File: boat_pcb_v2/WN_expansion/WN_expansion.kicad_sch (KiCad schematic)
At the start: 3 parts, among them J16 TSW-108-07-F-D, J17 TSW-108-07-F-D, J18 TSW-108-07-F-D

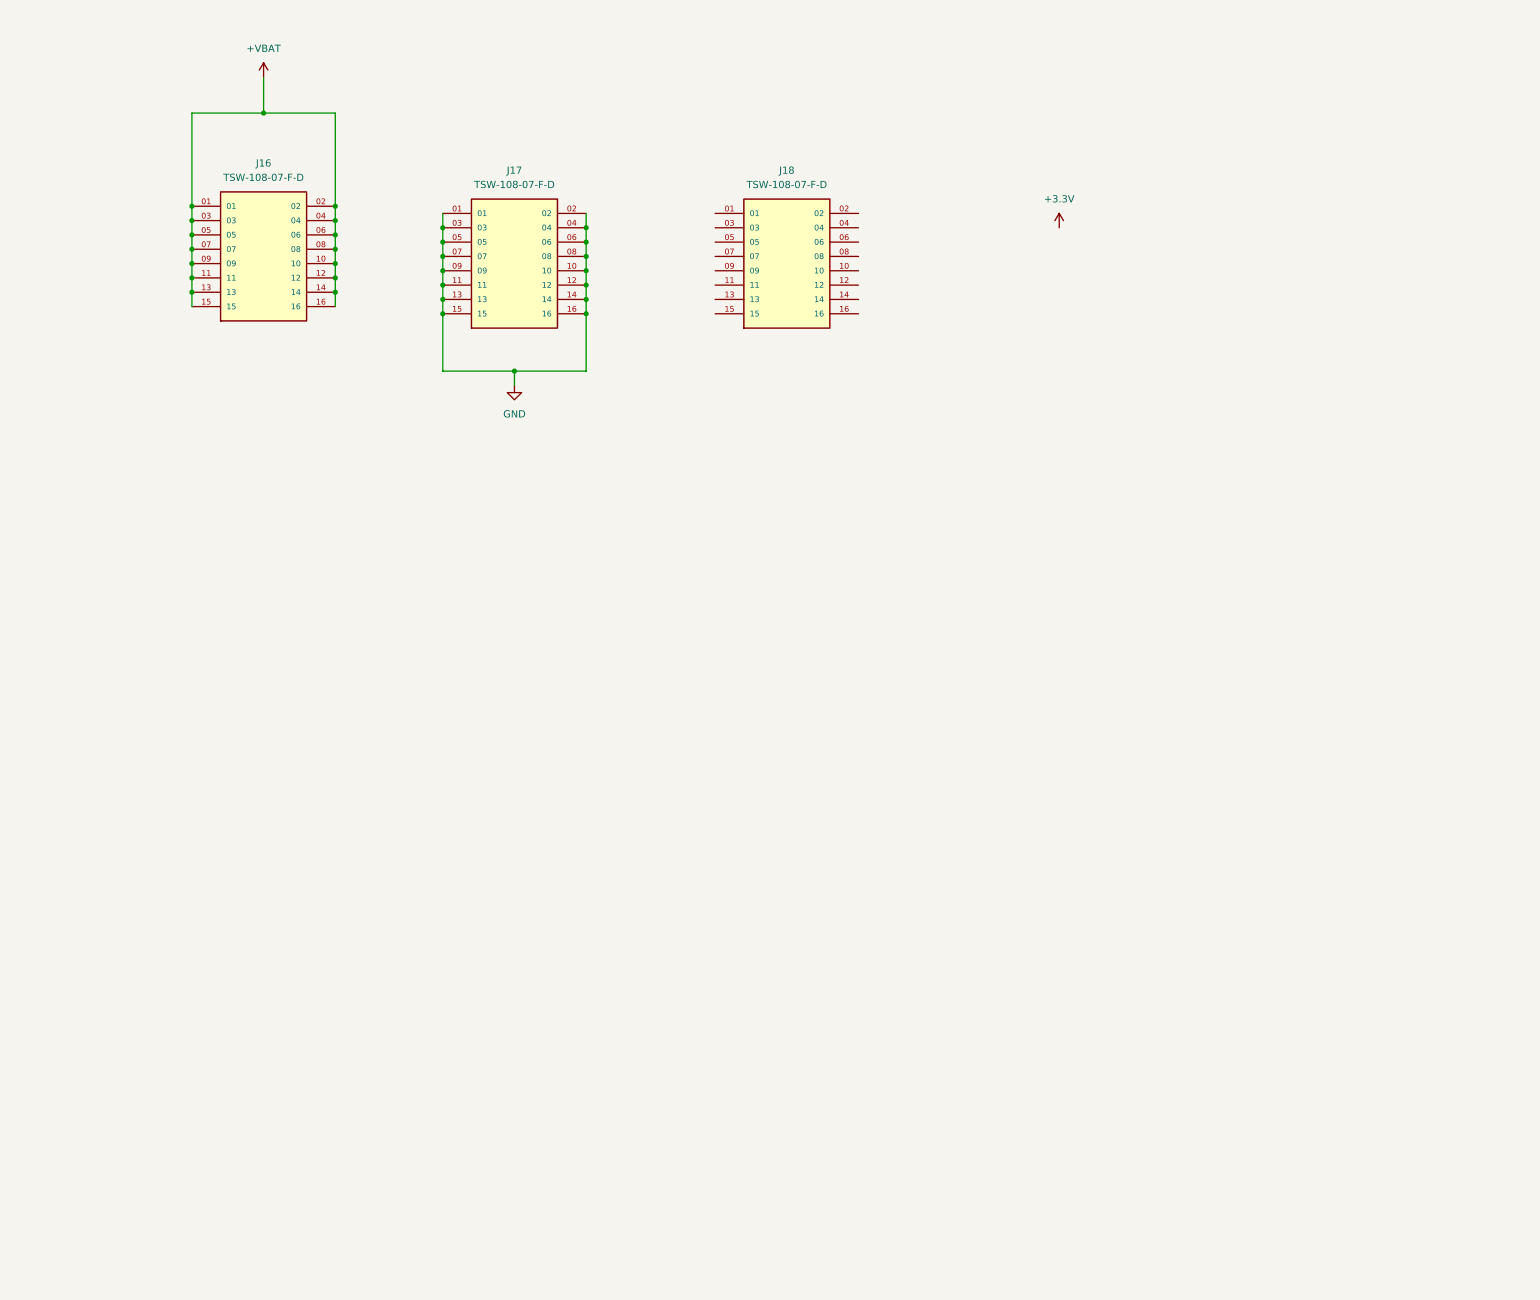
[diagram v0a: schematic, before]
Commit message: cleaned up expansion board
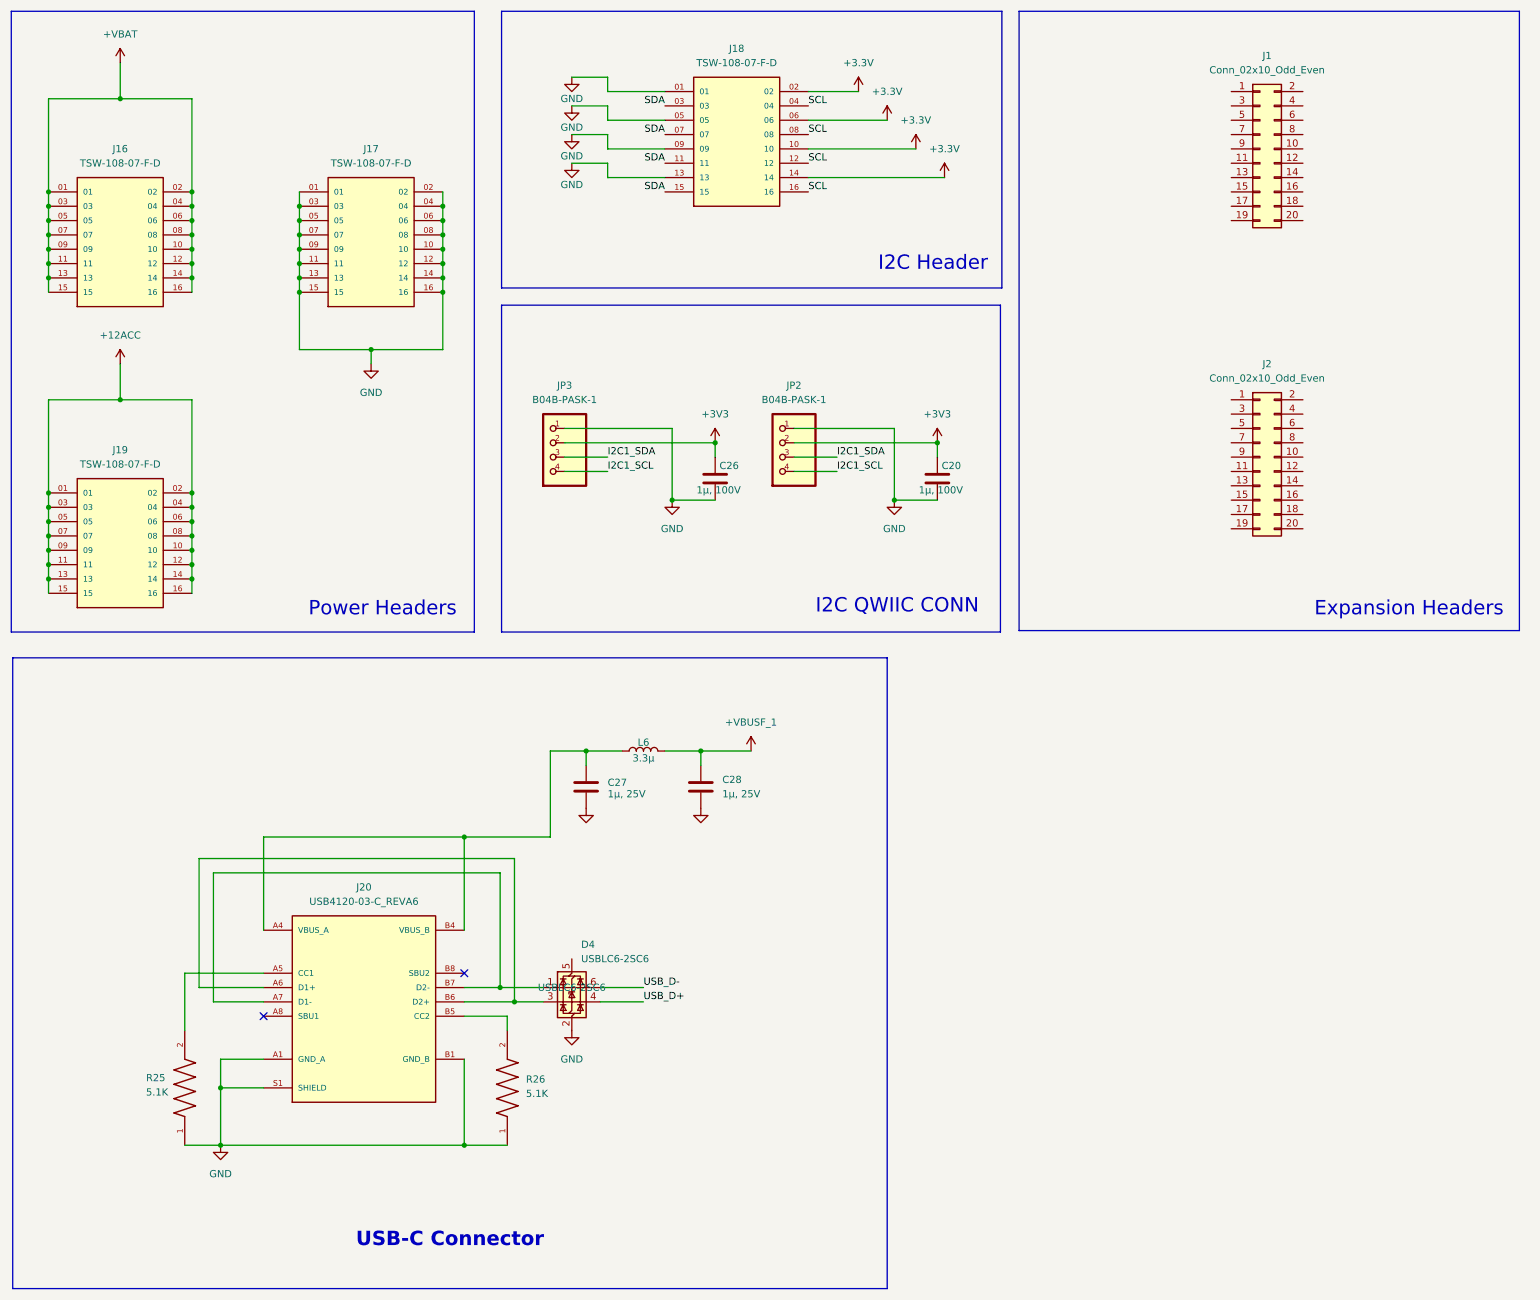
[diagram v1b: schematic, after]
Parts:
- added C20, C26: 1µ, 100V, WaterNet Footprints:CAPC2012X145N, symbol Device:C
- added C27, C28: 1µ, 25V, WaterNet26 Footprints:CAPC2012X145N, symbol Device:C
- added D4: USBLC6-2SC6, Package_TO_SOT_SMD:SOT-23-6, symbol Power_Protection:USBLC6-2SC6
- added J1, J2: Conn_02x10_Odd_Even, symbol Connector_Generic:Conn_02x10_Odd_Even
- added J19: TSW-108-07-F-D, WaterNet26 Library:SAMTEC_TSW-108-07-F-D, symbol WaterNet26 Library:TSW-108-07-F-D
- added J20: USB4120-03-C_REVA6, WaterNet26 Footprints:GCT_USB4120-03-C_REVA6, symbol WaterNet26 Library:USB4120-03-C_REVA6
- added JP2, JP3: B04B-PASK-1, WaterNet Footprints:B04B-PASK-1, symbol WaterNet Library:B04B-PASK-1_1
- added L6: 3.3µ, WaterNet26 Footprints:INDC1608X95N, symbol Device:L
- added R25, R26: 5.1K, WaterNet26 Footprints:RESC1508X55N, symbol WaterNet26 Library:RMCF0603FT5K10
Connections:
- net +3.3V: now also J18.02, J18.06, J18.10, J18.14
- net GND: now also J18.01, J18.05, J18.09, J18.13, C20.2, C26.2, C27.2, C28.2, D4.2 (GND), J20.A1 (GND_A), J20.A12 (GND_A), J20.B1 (GND_B), J20.B12 (GND_B), J20.S1 (SHIELD), J20.S2 (SHIELD), J20.S3 (SHIELD), J20.S4 (SHIELD), JP2.1, JP3.1, R25.1, R26.1
- net SDA: now reaches J18.03
- net SDA: now also J18.07, J18.11, J18.15
- net SCL: now reaches J18.04
- net SCL: now also J18.08, J18.12, J18.16
- new net: D4.1 (I/O1), J20.A7 (D1-), J20.B7 (D2-)
- new net: D4.3 (I/O2), J20.A6 (D1+), J20.B6 (D2+)
- new net: J20.A5 (CC1), R25.2
- new net: J20.B5 (CC2), R26.2
- new net +12ACC: J19.01, J19.02, J19.03, J19.04, J19.05, J19.06, J19.07, J19.08, J19.09, J19.10, J19.11, J19.12, J19.13, J19.14, J19.15, J19.16
- new net +3V3: C20.1, C26.1, JP2.2, JP3.2
- new net +VBUSF_1: C28.1, L6.2
- new net I2C1_SCL: JP2.4, JP3.4
- new net I2C1_SDA: JP2.3, JP3.3
- new net USB_D+: D4.4 (I/O2)
- new net USB_D-: D4.6 (I/O1)
- new net VBUS_A: C27.1, J20.A4 (VBUS_A), J20.A9 (VBUS_A), J20.B4 (VBUS_B), J20.B9 (VBUS_B), L6.1
- no-connect marks 0 -> 2
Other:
- note added: "Expansion Headers"
- note added: "I2C Header"
- note added: "I2C QWIIC CONN"
- note added: "Power Headers"
- note added: "USB-C Connector"
- moved on the sheet: J16, J17, J18
